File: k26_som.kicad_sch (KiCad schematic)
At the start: 49 parts, among them J6 22-23-2021, M1 XILINX-KRIA-K26, Q6 PJA3441, Q7 DTC014TEBTL

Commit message: Loclib of the project
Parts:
- R170: footprint antmicro-footprints:0402-res -> kria-k26-devboard-footprints:0402-res; symbol antmicroResistors0402:R_0R_0402 -> kria-k26-devboard:R_0R_0402

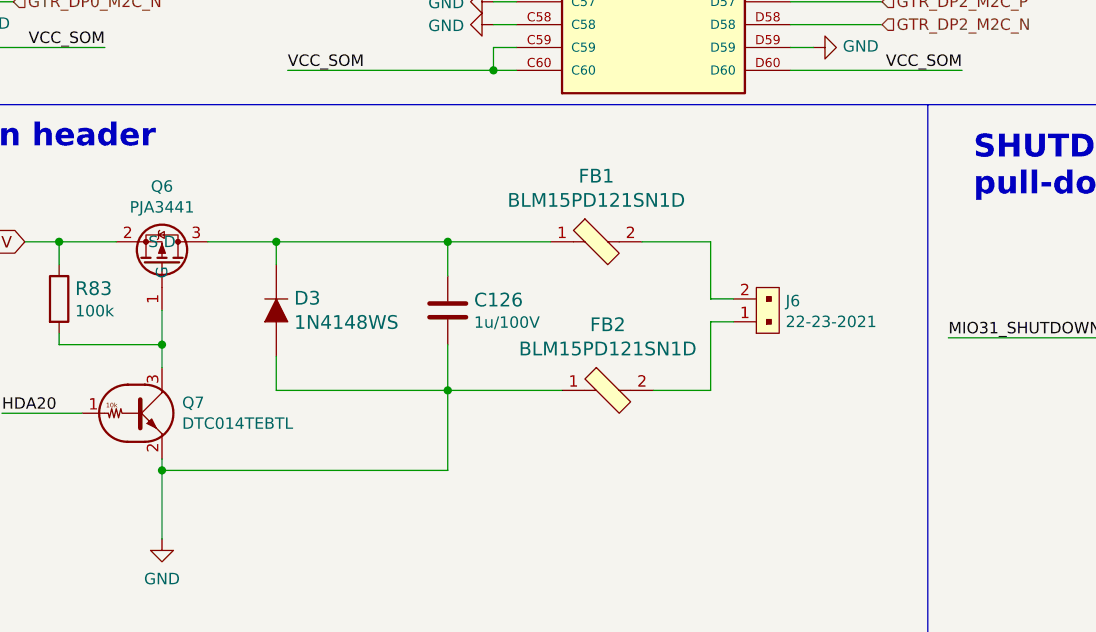
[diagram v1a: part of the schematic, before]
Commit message: Bom optimization
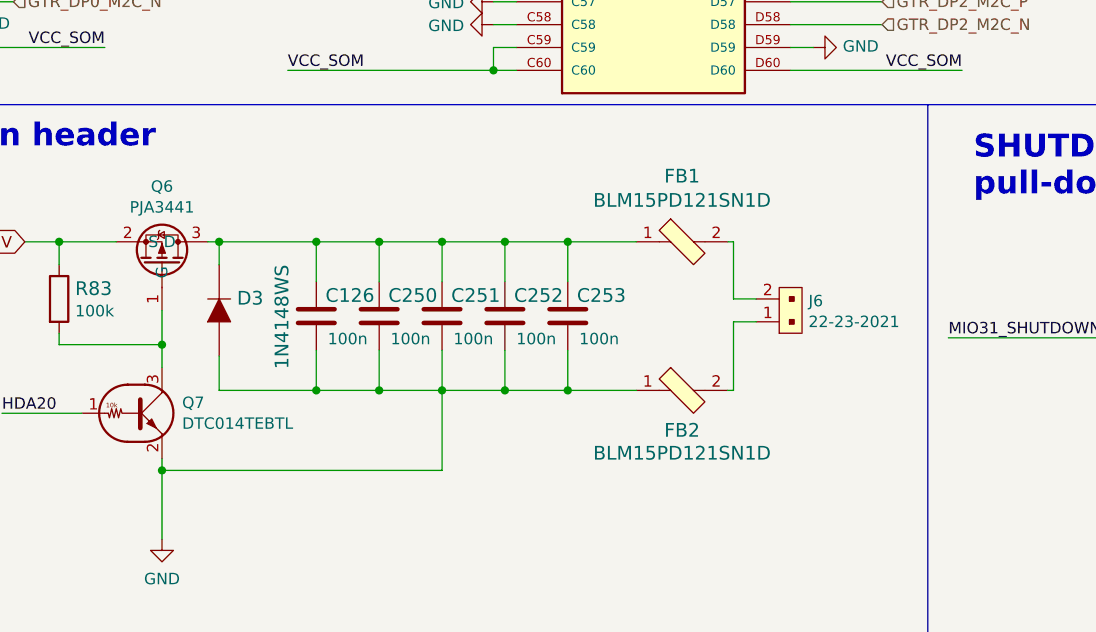
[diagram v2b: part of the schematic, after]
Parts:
- removed C126: C_1u_1210_100V, kria-k26-devboard-footprints:1210-cap, symbol kria-k26-devboard:C_1u_1210_100V
- added C126, C250, C251, C252, C253: C_100n_0402, kria-k26-devboard-footprints:0402-cap, symbol kria-k26-devboard:C_100n_0402
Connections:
- net GND: now also C126.2, C250.2, C251.2, C252.2, C253.2
- net at D3.K, FB1.1, Q6.3 (D): now also C126.1, C250.1, C251.1, C252.1, C253.1
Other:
- moved on the sheet: D3, FB1, FB2, J6
